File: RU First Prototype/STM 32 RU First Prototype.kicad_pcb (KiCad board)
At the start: 4 copper layers, 60.8 x 74.2 mm, 95 parts, among them J1 Conn_01x02, J10 Conn_01x02_Pin, J11 Conn_01x02_Pin, J12 1776113-2, J2 USB_C_Receptacle, J3 Conn_01x02_Pin, J4 Conn_01x04, J5 Conn_01x02_Pin, J7 1776113-2, J9 Conn_01x02_Pin, Q1 SISA96DN-T1, Q3 SISA96DN-T1, SW1 SW_SPDT, U1 STM32F412RGTx, U2 AMS1117-3.3, U3 MS5611, U4 KX134-1211, U5 W25Q16JVSS, U6 TCAN330, U7 TCAN330, Y1 Crystal_8Mhz

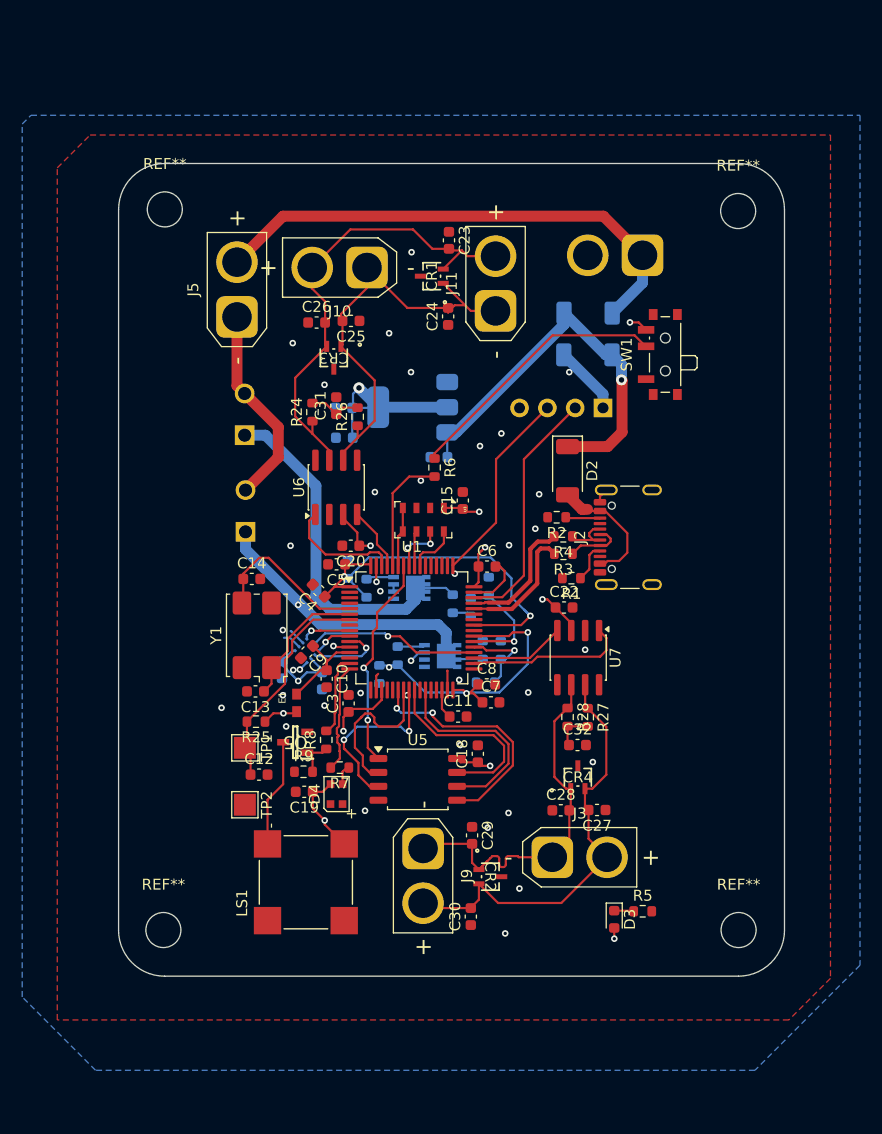
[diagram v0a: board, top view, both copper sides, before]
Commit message: Made some changes
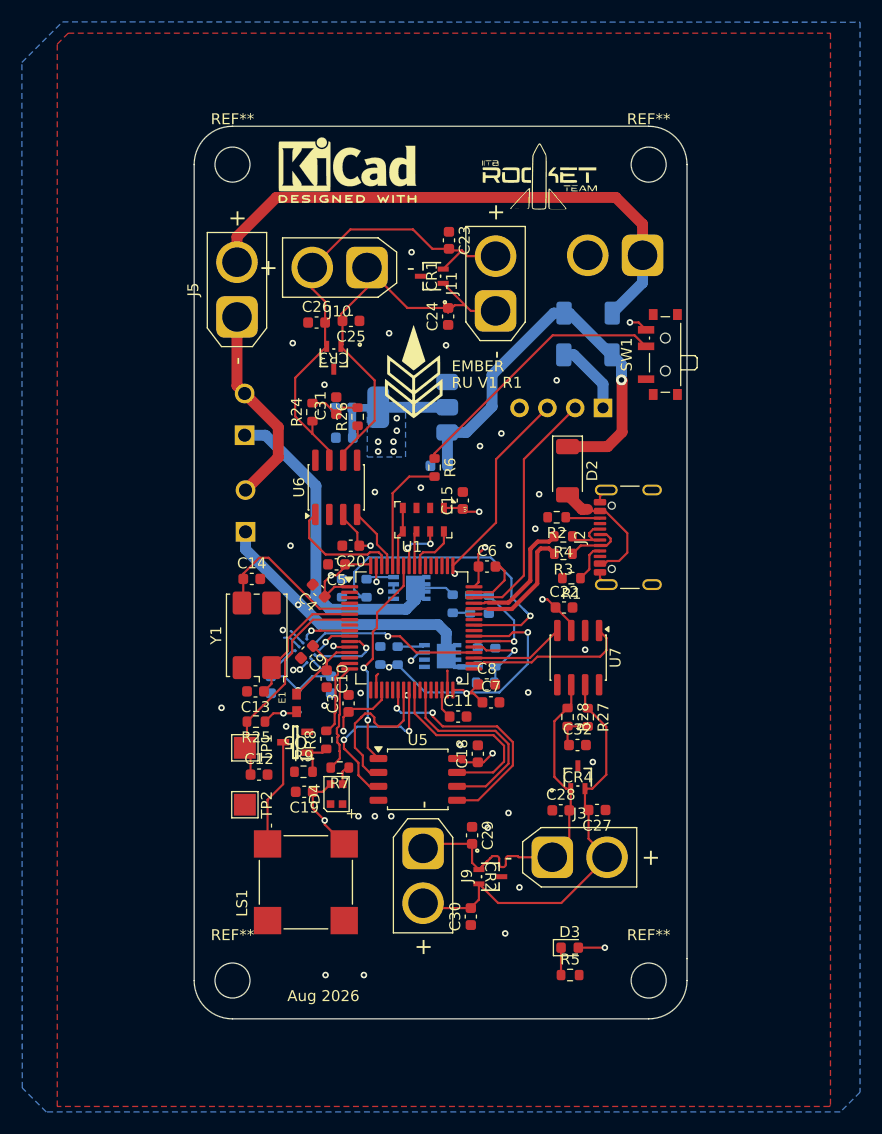
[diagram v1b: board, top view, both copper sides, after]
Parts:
- added G***: LOGO, RT_Graphics:RT_logo, F.Cu at (133.0, 59.0)
- added G***: LOGO, RT_Graphics:Ember_logo, F.Cu at (121.5, 76.5)
- added REF**: KiCad-Logo2_5mm_SilkScreen, Symbol:KiCad-Logo2_5mm_SilkScreen, F.Cu at (115.5, 58.0)
- moved REF** 9.42 mm to (143.0, 132.0)
- moved REF** 9.20 mm to (143.0, 57.5)
- moved R5 8.82 mm to (135.8, 131.5)
- moved REF** 7.81 mm to (105.0, 132.0)
- moved REF** 7.41 mm to (105.0, 57.5)
- moved D3 4.82 mm to (135.8, 129.0), turned to 0 degrees
- moved R11 1.81 mm to (115.0, 96.2)
- moved R14 1.73 mm to (118.5, 102.3), turned to -90 degrees
- moved C17 1.71 mm to (108.5, 105.0)
- moved R20 1.67 mm to (128.4, 97.7), turned to -90 degrees
- moved C16 0.90 mm to (114.0, 105.0)
- moved R22 0.82 mm to (129.0, 102.5)
- moved C1 0.79 mm to (123.8, 85.0)
- moved R21 0.75 mm to (127.4, 102.4)
- moved R19 0.28 mm to (126.7, 97.6)
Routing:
- net /V_2S: track 47.7 -> 52.2 mm
- net +3V3: track 76.5 -> 79.8 mm, vias 14 -> 19
- net /Main: track 29.4 -> 31.4 mm
- net /V_IN: track 38.0 -> 39.8 mm
- net GND: track 19.4 -> 20.8 mm, vias 40 -> 44
- net /V_DROGUE: track 28.5 -> 27.3 mm
- net Net-(D3-K): track 1.80 -> 2.50 mm
- net /SW_VCC: track 6.33 -> 6.87 mm
- added copper zone on B.Cu, net +3V3
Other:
- board size 60.8 x 74.2 mm -> 45 x 81.5 mm
- board text added: "Aug 2026"
- board text added: "EMBER"
- board text added: "RU V1 R1"
